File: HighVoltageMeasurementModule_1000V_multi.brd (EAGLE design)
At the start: 48 x 24 mm, 31 parts, among them X1 MKDSN1,5/2-5,08, X2 MKDSN1,5/2-5,08

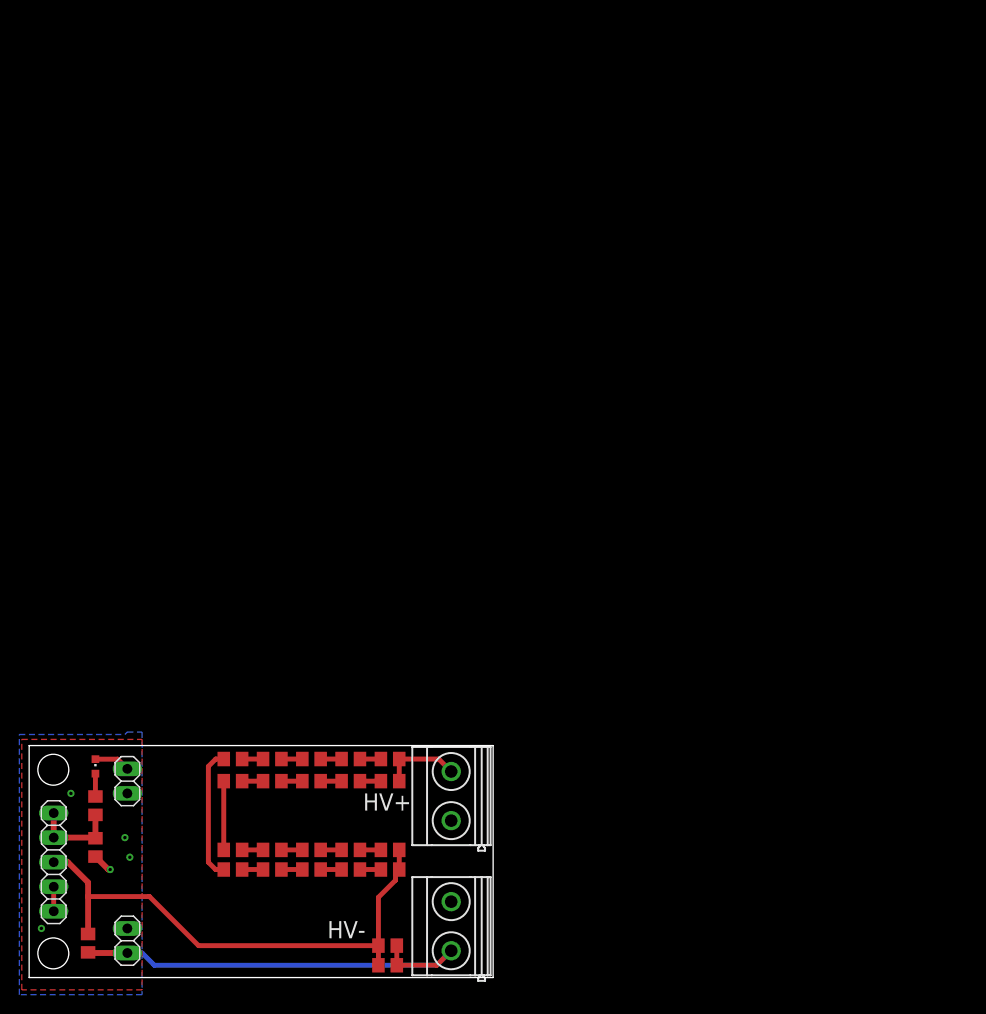
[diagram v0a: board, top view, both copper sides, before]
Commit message: multiversion finished
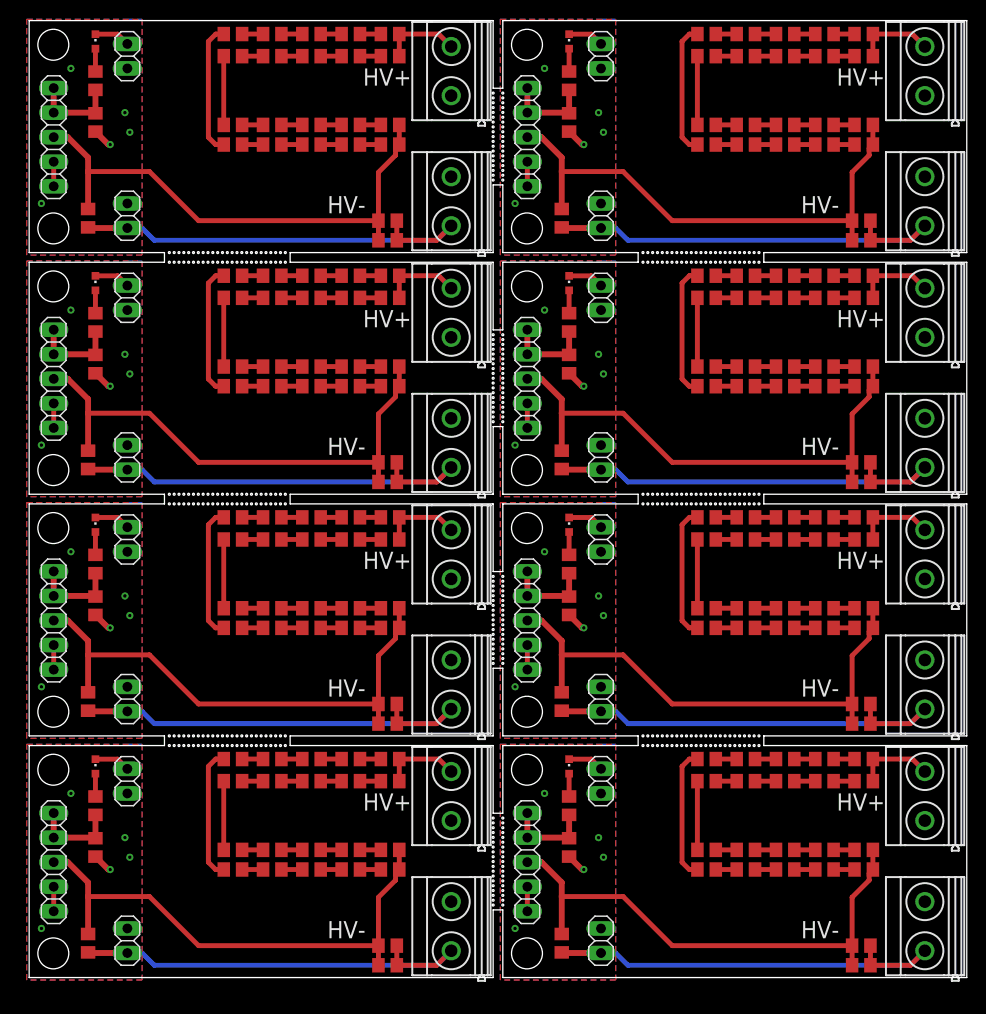
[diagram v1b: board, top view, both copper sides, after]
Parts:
- added C10, C12, C14, C16, C18, C6, C8: 10nF, rcl:C0805
- added C11, C13, C15, C17, C5, C7, C9: 100nF, rcl:C0805
- added JP10, JP13, JP16, JP19, JP22, JP25, JP7: (no value), pinhead:1X05
- added JP11, JP12, JP14, JP15, JP17, JP18, JP20, JP21, JP23, JP24, JP26, JP27, JP8, JP9: (no value), pinhead:1X02
- added LED3, LED4, LED5, LED6, LED7, LED8, LED9: KT-0603R, led:CHIPLED_0603
- added R100, R101, R102, R103, R105, R106, R107, R108, R109, R110, R111, R112, R113, R114, R117, R118, R119, R120, R121, R122, R123, R124, R125, R126, R128, R129, R130, R131, R132, R133, R134, R135, R136, R137, R140, R141, R142, R143, R144, R145, R146, R147, R148, R149, R151, R152, R153, R154, R155, R156, R157, R158, R159, R160, R163, R164, R165, R166, R167, R168, R169, R170, R171, R172, R174, R175, R176, R177, R178, R179, R180, R181, R182, R183, R186, R187, R188, R189, R190, R191, R192, R193, R194, R195, R197, R198, R199, R200, R201, R202, R203, R204, R205, R206, R47, R48, R49, R50, R51, R52, R54, R55, R56, R57, R59, R60, R61, R62, R63, R64, R65, R66, R67, R68, R71, R72, R73, R74, R75, R76, R77, R78, R79, R80, R82, R83, R84, R85, R86, R87, R88, R89, R90, R91, R94, R95, R96, R97, R98, R99: 200k, rcl:R0805
- added R104, R115, R127, R138, R150, R161, R173, R184, R196, R207, R58, R69, R81, R92: 10k, rcl:R0805
- added R116, R139, R162, R185, R46, R70, R93: 1k, rcl:R0805
- added X10, X11, X12, X13, X14, X15, X16, X17, X18, X5, X6, X7, X8, X9: MKDSN1,5/2-5,08, con-phoenix-508:MKDSN1,5/2-5,08
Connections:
- new net N$100: C10.2, JP13.3, R103.2, R104.2, R114.2, R115.2
- new net N$101: LED6.A, R116.2
- new net N$102: R117.2, R118.1
- new net N$103: R118.2, R119.1
- new net N$104: R119.2, R120.1
- new net N$105: R120.2, R121.1
- new net N$106: R121.2, R122.1
- new net N$107: R122.2, R123.1
- new net N$108: R123.2, R124.1
- new net N$109: R124.2, R125.1
- new net N$110: R125.2, R126.1
- new net N$111: R128.2, R129.1
- new net N$112: R129.2, R130.1
- new net N$113: R130.2, R131.1
- new net N$114: R131.2, R132.1
- new net N$115: R132.2, R133.1
- new net N$116: R133.2, R134.1
- new net N$117: R134.2, R135.1
- new net N$118: R135.2, R136.1
- new net N$119: R136.2, R137.1
- new net N$120: C12.2, JP16.3, R126.2, R127.2, R137.2, R138.2
- new net N$121: LED7.A, R139.2
- new net N$122: R140.2, R141.1
- new net N$123: R141.2, R142.1
- new net N$124: R142.2, R143.1
- new net N$125: R143.2, R144.1
- new net N$126: R144.2, R145.1
- new net N$127: R145.2, R146.1
- new net N$128: R146.2, R147.1
- new net N$129: R147.2, R148.1
- new net N$130: R148.2, R149.1
- new net N$131: R151.2, R152.1
- new net N$132: R152.2, R153.1
- new net N$133: R153.2, R154.1
- new net N$134: R154.2, R155.1
- new net N$135: R155.2, R156.1
- new net N$136: R156.2, R157.1
- new net N$137: R157.2, R158.1
- new net N$138: R158.2, R159.1
- new net N$139: R159.2, R160.1
- new net N$140: C14.2, JP19.3, R149.2, R150.2, R160.2, R161.2
- new net N$141: LED8.A, R162.2
- new net N$142: R163.2, R164.1
- new net N$143: R164.2, R165.1
- new net N$144: R165.2, R166.1
- new net N$145: R166.2, R167.1
- new net N$146: R167.2, R168.1
- new net N$147: R168.2, R169.1
- new net N$148: R169.2, R170.1
- new net N$149: R170.2, R171.1
- new net N$150: R171.2, R172.1
- new net N$151: R174.2, R175.1
- new net N$152: R175.2, R176.1
- new net N$153: R176.2, R177.1
- new net N$154: R177.2, R178.1
- new net N$155: R178.2, R179.1
- new net N$156: R179.2, R180.1
- new net N$157: R180.2, R181.1
- new net N$158: R181.2, R182.1
- new net N$159: R182.2, R183.1
- new net N$160: C16.2, JP22.3, R172.2, R173.2, R183.2, R184.2
- new net N$161: LED9.A, R185.2
- new net N$162: R186.2, R187.1
- new net N$163: R187.2, R188.1
- new net N$164: R188.2, R189.1
- new net N$165: R189.2, R190.1
- new net N$166: R190.2, R191.1
- new net N$167: R191.2, R192.1
- new net N$168: R192.2, R193.1
- new net N$169: R193.2, R194.1
- new net N$170: R194.2, R195.1
- new net N$171: R197.2, R198.1
- new net N$172: R198.2, R199.1
- new net N$173: R199.2, R200.1
- new net N$174: R200.2, R201.1
- new net N$175: R201.2, R202.1
- new net N$176: R202.2, R203.1
- new net N$177: R203.2, R204.1
- new net N$178: R204.2, R205.1
- new net N$179: R205.2, R206.1
- new net N$180: C18.2, JP25.3, R195.2, R196.2, R206.2, R207.2
- new net N$40: LED3.A, R46.2
- new net N$42: R47.2, R48.1
- new net N$43: R48.2, R49.1
- new net N$44: R49.2, R50.1
- new net N$45: R50.2, R51.1
- new net N$46: R51.2, R52.1
- new net N$47: R52.2, R54.1
- new net N$48: R54.2, R55.1
- new net N$49: R55.2, R56.1
- new net N$50: R56.2, R57.1
- new net N$51: R59.2, R60.1
- new net N$52: R60.2, R61.1
- new net N$53: R61.2, R62.1
- new net N$54: R62.2, R63.1
- new net N$55: R63.2, R64.1
- new net N$56: R64.2, R65.1
- new net N$57: R65.2, R66.1
- new net N$58: R66.2, R67.1
- new net N$59: R67.2, R68.1
- new net N$60: C6.2, JP7.3, R57.2, R58.2, R68.2, R69.2
- new net N$61: LED4.A, R70.2
- new net N$62: R71.2, R72.1
- new net N$63: R72.2, R73.1
- new net N$64: R73.2, R74.1
- new net N$65: R74.2, R75.1
- new net N$66: R75.2, R76.1
- new net N$67: R76.2, R77.1
- new net N$68: R77.2, R78.1
- new net N$69: R78.2, R79.1
- new net N$70: R79.2, R80.1
- new net N$71: R82.2, R83.1
- new net N$72: R83.2, R84.1
- new net N$73: R84.2, R85.1
- new net N$74: R85.2, R86.1
- new net N$75: R86.2, R87.1
- new net N$76: R87.2, R88.1
- new net N$77: R88.2, R89.1
- new net N$78: R89.2, R90.1
- new net N$79: R90.2, R91.1
- new net N$80: C8.2, JP10.3, R80.2, R81.2, R91.2, R92.2
- new net N$81: LED5.A, R93.2
- new net N$82: R94.2, R95.1
- new net N$83: R95.2, R96.1
- new net N$84: R96.2, R97.1
- new net N$85: R97.2, R98.1
- new net N$86: R98.2, R99.1
- new net N$87: R100.1, R99.2
- new net N$88: R100.2, R101.1
- new net N$89: R101.2, R102.1
- new net N$90: R102.2, R103.1
- new net N$91: R105.2, R106.1
- new net N$92: R106.2, R107.1
- new net N$93: R107.2, R108.1
- new net N$94: R108.2, R109.1
- new net N$95: R109.2, R110.1
- new net N$96: R110.2, R111.1
- new net N$97: R111.2, R112.1
- new net N$98: R112.2, R113.1
- new net N$99: R113.2, R114.1
- net 5VDC: now also C11.2, C13.2, C15.2, C17.2, C5.2, C7.2, C9.2, JP10.1, JP10.2, JP13.1, JP13.2, JP16.1, JP16.2, JP19.1, JP19.2, JP22.1, JP22.2, JP25.1, JP25.2, JP7.1, JP7.2, R116.1, R139.1, R162.1, R185.1, R46.1, R70.1, R93.1
- net GND: now also C10.1, C11.1, C12.1, C13.1, C14.1, C15.1, C16.1, C17.1, C18.1, C5.1, C6.1, C7.1, C8.1, C9.1, JP10.4, JP10.5, JP11.1, JP11.2, JP12.1, JP12.2, JP13.4, JP13.5, JP14.1, JP14.2, JP15.1, JP15.2, JP16.4, JP16.5, JP17.1, JP17.2, JP18.1, JP18.2, JP19.4, JP19.5, JP20.1, JP20.2, JP21.1, JP21.2, JP22.4, JP22.5, JP23.1, JP23.2, JP24.1, JP24.2, JP25.4, JP25.5, JP26.1, JP26.2, JP27.1, JP27.2, JP7.4, JP7.5, JP8.1, JP8.2, JP9.1, JP9.2, LED3.C, LED4.C, LED5.C, LED6.C, LED7.C, LED8.C, LED9.C, R104.1, R115.1, R127.1, R138.1, R150.1, R161.1, R173.1, R184.1, R196.1, R207.1, R58.1, R69.1, R81.1, R92.1, X10.1, X12.1, X14.1, X16.1, X18.1, X6.1, X8.1
- net HV+: now also R105.1, R117.1, R128.1, R140.1, R151.1, R163.1, R174.1, R186.1, R197.1, R47.1, R59.1, R71.1, R82.1, R94.1, X11.2, X13.2, X15.2, X17.2, X5.2, X7.2, X9.2
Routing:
- net GND: track 55.4 -> 442.9 mm, vias 5 -> 40
- net 5VDC: track 9.30 -> 74.4 mm
- net HV+: track 8.20 -> 65.6 mm
- net N$180: track 0.00 -> 54.7 mm
- net N$140: track 0.00 -> 54.7 mm
- net N$100: track 0.00 -> 54.7 mm
- net N$160: track 0.00 -> 54.7 mm
- net N$120: track 0.00 -> 54.7 mm
- net N$80: track 0.00 -> 54.7 mm
- net N$60: track 0.00 -> 54.7 mm
- net N$86: track 0.00 -> 13.7 mm
- net N$126: track 0.00 -> 13.7 mm
- net N$166: track 0.00 -> 13.7 mm
- net N$146: track 0.00 -> 13.7 mm
- net N$46: track 0.00 -> 13.7 mm
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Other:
- board size 48 x 24 mm -> 97 x 99 mm
